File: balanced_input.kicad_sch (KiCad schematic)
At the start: 4 parts

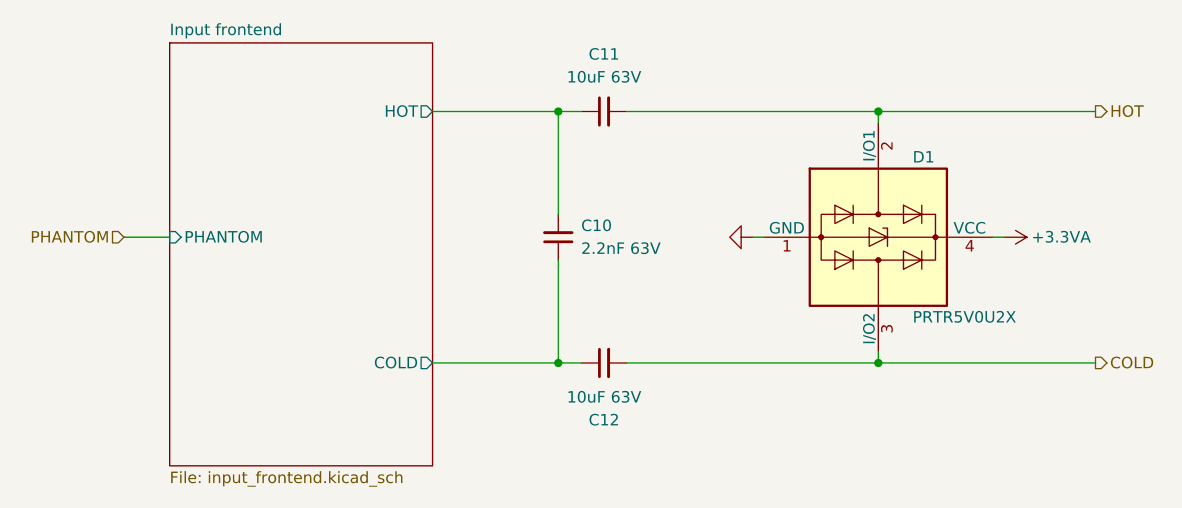
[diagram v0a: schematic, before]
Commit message: update component assignments
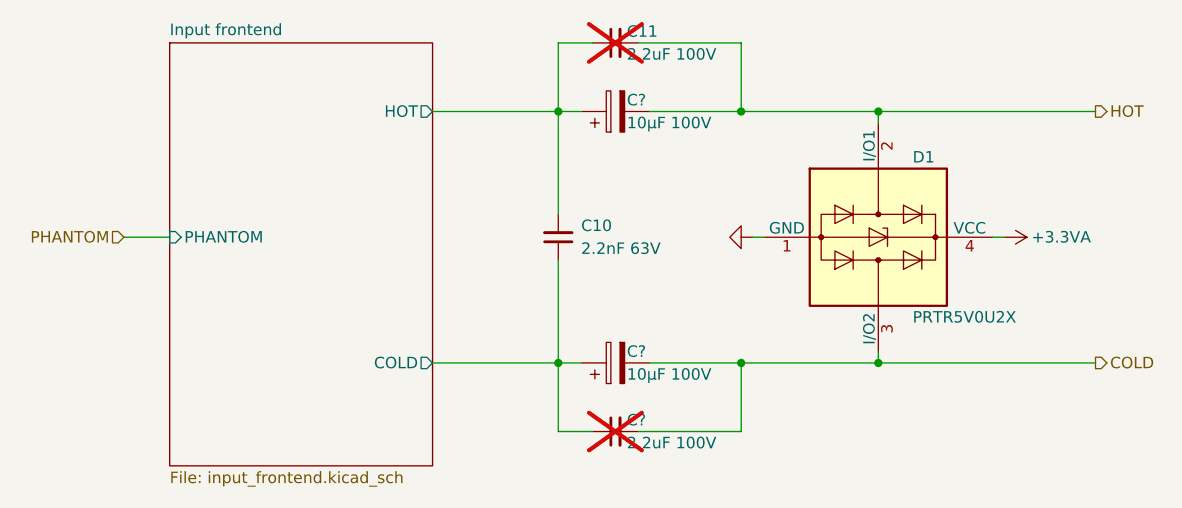
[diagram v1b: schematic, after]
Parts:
- removed C12: 10uF 63V, Capacitor_SMD:C_0603_1608Metric, symbol Device:C_Small
- added C? (x2): 10μF 100V, Capacitor_THT:CP_Radial_D5.0mm_P2.00mm, symbol Device:C_Polarized
- added C?: 2.2uF 100V, Capacitor_SMD:C_1206_3216Metric, symbol Device:C_Small
- C10: MPN C 2.2nF 63V 0805 -> C 2.2nF 63V 0603
- C11: value 10uF 63V -> 2.2uF 100V; footprint Capacitor_SMD:C_0603_1608Metric -> Capacitor_SMD:C_1206_3216Metric; MPN C 10μF 63V 0805 -> C 2.2μF 100V 1206; now not fitted
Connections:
- net COLD: now also C?.2, C?.2
- net HOT: now also C?.2
- net Input frontend/COLD: now also C?.1, C?.1
- net Input frontend/HOT: now also C?.1

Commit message: sync pcb
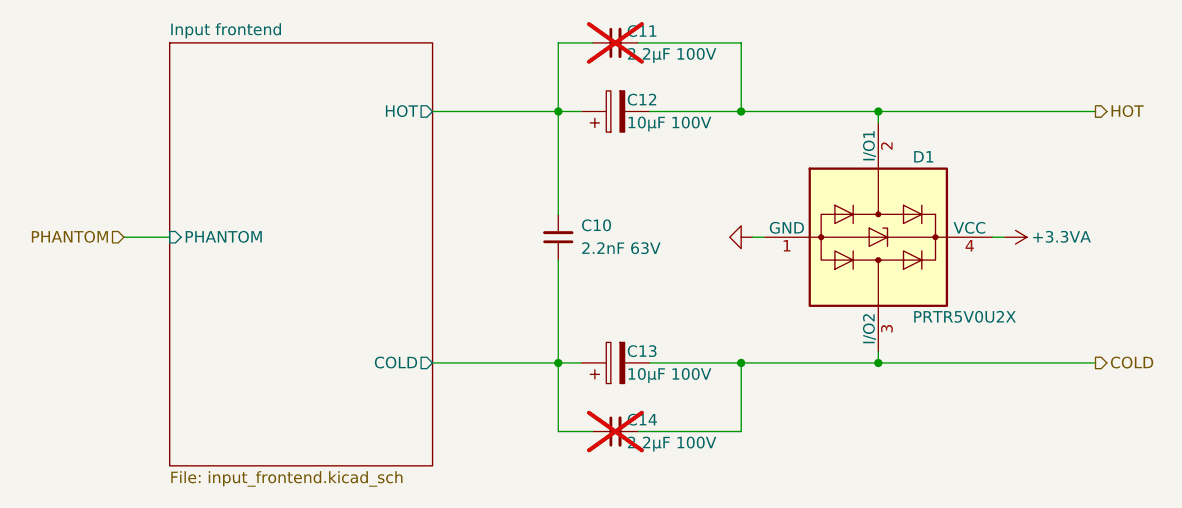
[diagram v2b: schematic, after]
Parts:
- C11: value 2.2uF 100V -> 2.2μF 100V
- C14: renamed from C?; value 2.2uF 100V -> 2.2μF 100V
- gave numbers to parts that had none: 2
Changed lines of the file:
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@@
 		(on_board yes)
 		(dnp no)
-		(property "Reference" "C?"
+		(property "Reference" "C13"
 			(at 153.67 91.44 90)
 			(effects
@@
 			(project "mv2_taa3040"
 				(path "/41a55a1d-5108-482f-b313-9eaa5d011dff/e3f94415-cffd-4131-bc0e-4234c6300c0c"
-					(reference "C?")
-					(unit 1)
-				)
-				(path "/41a55a1d-5108-482f-b313-9eaa5d011dff/ec88f180-6d4b-439f-8697-a1ff92f435a7"
-					(reference "C?")
+					(reference "C13")
+					(unit 1)
+				)
+				(path "/41a55a1d-5108-482f-b313-9eaa5d011dff/ec88f180-6d4b-439f-8697-a1ff92f435a7"
+					(reference "C18")
 					(unit 1)
 				)
@@
 		(on_board yes)
 		(dnp no)
-		(property "Reference" "C?"
+		(property "Reference" "C12"
 			(at 153.67 63.5 90)
 			(effects
@@
 			(project ""
 				(path "/41a55a1d-5108-482f-b313-9eaa5d011dff/e3f94415-cffd-4131-bc0e-4234c6300c0c"
-					(reference "C?")
+					(reference "C12")
+					(unit 1)
+				)
+				(path "/41a55a1d-5108-482f-b313-9eaa5d011dff/ec88f180-6d4b-439f-8697-a1ff92f435a7"
+					(reference "C17")
 					(unit 1)
 				)
@@
 				)
 				(path "/41a55a1d-5108-482f-b313-9eaa5d011dff/ec88f180-6d4b-439f-8697-a1ff92f435a7"
-					(reference "C13")
+					(reference "C15")
 					(unit 1)
 				)
@@
 			)
 		)
-		(property "Value" "2.2uF 100V"
+		(property "Value" "2.2μF 100V"
 			(at 153.67 58.42 90)
 			(effects
@@
 				)
 				(path "/41a55a1d-5108-482f-b313-9eaa5d011dff/ec88f180-6d4b-439f-8697-a1ff92f435a7"
-					(reference "C14")
+					(reference "C16")
 					(unit 1)
 				)
@@
 		(on_board yes)
 		(dnp yes)
-		(property "Reference" "C?"
+		(property "Reference" "C14"
 			(at 153.67 99.06 90)
 			(effects
@@
 			)
 		)
-		(property "Value" "2.2uF 100V"
+		(property "Value" "2.2μF 100V"
 			(at 153.67 101.6 90)
 			(effects
@@
 			(project "mv2_taa3040"
 				(path "/41a55a1d-5108-482f-b313-9eaa5d011dff/e3f94415-cffd-4131-bc0e-4234c6300c0c"
-					(reference "C?")
-					(unit 1)
-				)
-				(path "/41a55a1d-5108-482f-b313-9eaa5d011dff/ec88f180-6d4b-439f-8697-a1ff92f435a7"
-					(reference "C?")
-					(unit 1)
-				)
+					(reference "C14")
+					(unit 1)
+				)
+				(path "/41a55a1d-5108-482f-b313-9eaa5d011dff/ec88f180-6d4b-439f-8697-a1ff92f435a7"
+					(reference "C19")
+					(unit 1)
+				)
